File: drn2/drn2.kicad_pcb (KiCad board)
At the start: 2 copper layers, 123 x 89 mm, 60 parts, among them J1 Conn_01x03_Socket, J12 Conn_01x03_Socket, J13 Conn_01x03_Socket, J14GND1 Conn_01x03_Socket, J15VBECOUT1 Conn_01x03_Socket, J16 Conn_01x03_Socket, J2 Raspberry_Pi_2_3, J3 Conn_01x03_Socket, J3_F1_BEC_OUT1 Conn_01x02_Pin, J3_F2_BAT1 Conn_01x02_Pin, J4 Conn_01x03_Socket, J4_M0_MOT0 Conn_01x02_Pin, J4_M1_MOT1 Conn_01x02_Pin, J4_M2_MOT2 Conn_01x02_Pin, J4_M3_MOT3 Conn_01x02_Pin, J4_M4_BEC_IN1 Conn_01x02_Pin, J5 Conn_01x12_Socket, J6 Conn_01x08_Socket, J7 Conn_01x03_Socket, J8 Conn_01x03_Socket, U1 LSM9DS1, Y1 TestPoint

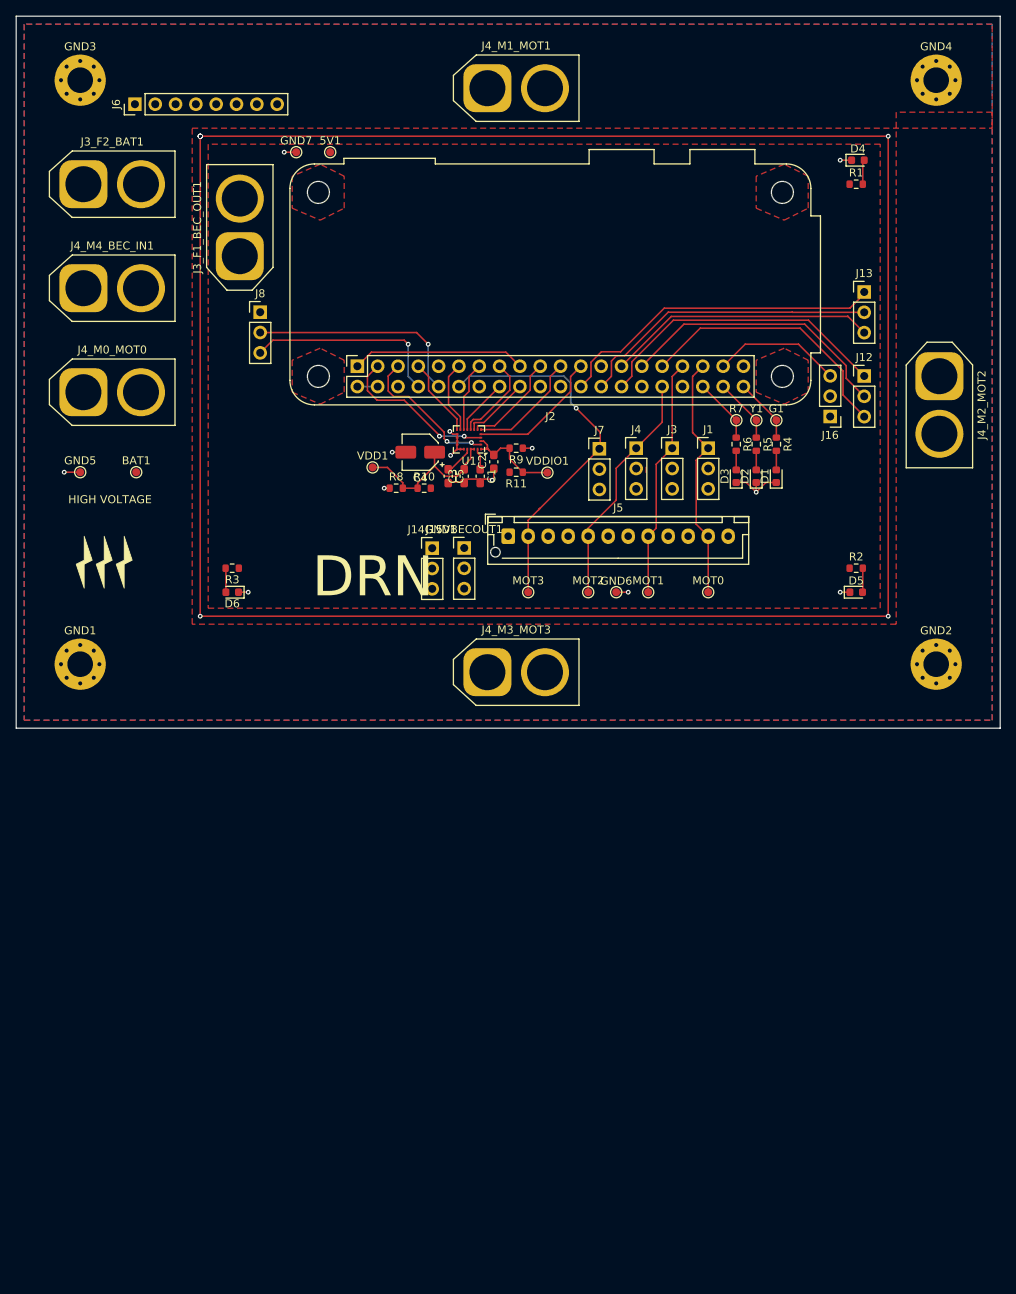
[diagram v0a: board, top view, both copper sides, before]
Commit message: feat: drn pcb v3 almost done
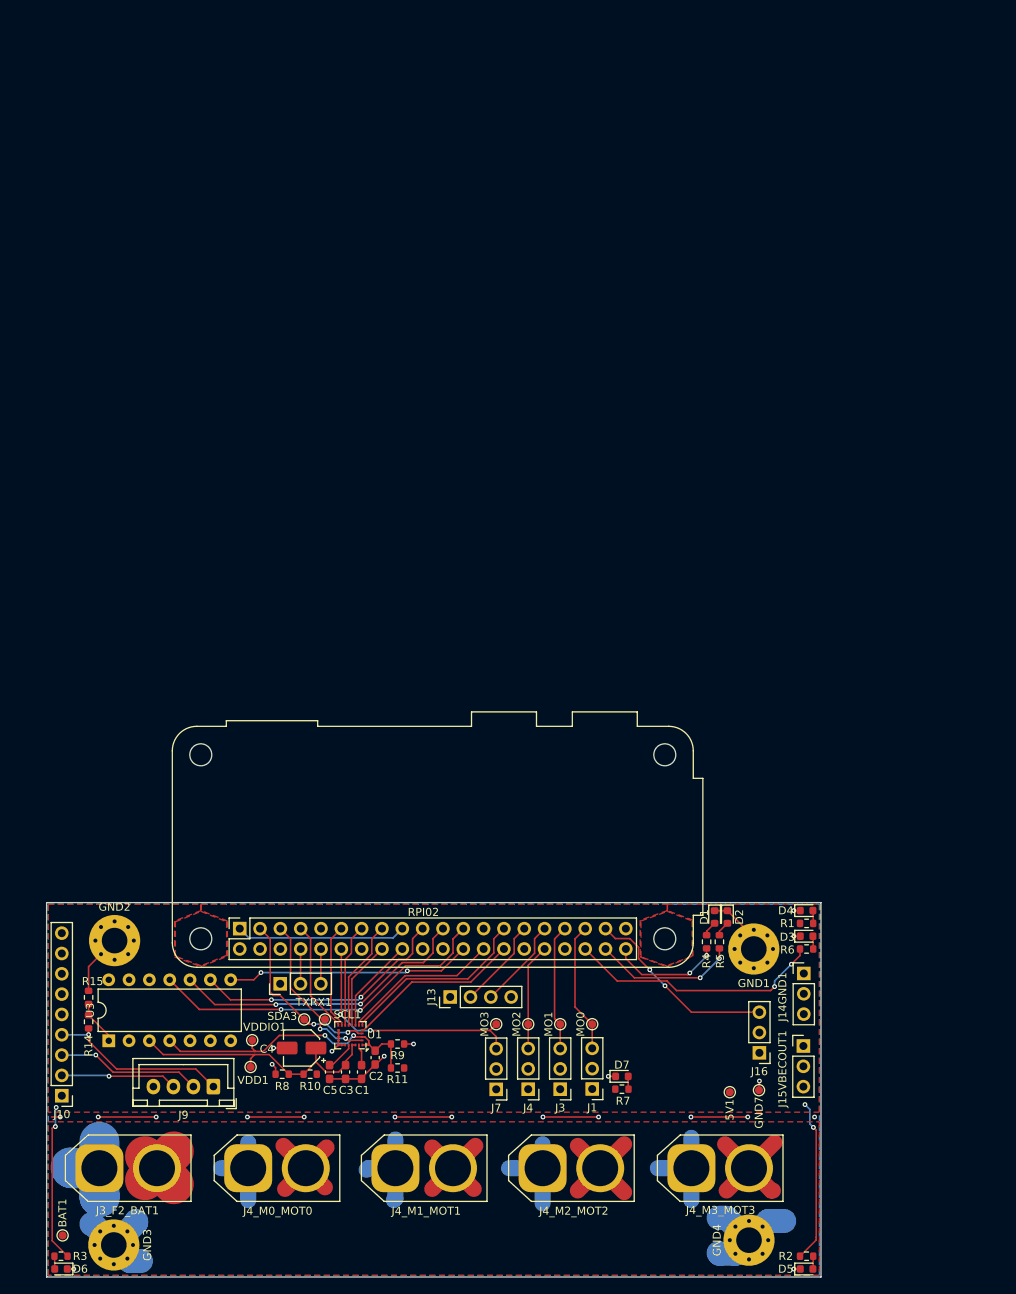
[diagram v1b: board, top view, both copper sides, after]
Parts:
- removed G1, GND5, GND6, MOT0, MOT1, MOT2, MOT3, Y1: TestPoint, TestPoint:TestPoint_Pad_D1.0mm
- removed J12, J8: Conn_01x03_Socket, Connector_PinHeader_2.54mm:PinHeader_1x03_P2.54mm_Vertical
- removed J2: Raspberry_Pi_2_3, Module:Raspberry_Pi_Zero_Socketed_THT_FaceDown_MountingHoles
- removed J3_F1_BEC_OUT1, J4_M4_BEC_IN1: Conn_01x02_Pin, Connector_AMASS:AMASS_XT60-F_1x02_P7.20mm_Vertical
- removed J5: Conn_01x12_Socket, Connector_JST:JST_XH_B12B-XH-AM_1x12_P2.50mm_Vertical
- removed J6: Conn_01x08_Socket, Connector_PinHeader_2.54mm:PinHeader_1x08_P2.54mm_Vertical
- added D7: LEDI, LED_SMD:LED_0603_1608Metric, F.Cu at (134.7, 158.5)
- added J10: Conn_01x09_Socket, Connector_PinHeader_2.54mm:PinHeader_1x09_P2.54mm_Vertical, F.Cu at (64.7, 160.9)
- added J9: Conn_01x04_Pin, Connector_JST:JST_XH_B4B-XH-A_1x04_P2.50mm_Vertical, F.Cu at (83.7, 159.8)
- added MO0: TestPoint, TestPoint:TestPoint_Pad_D1.0mm, F.Cu at (131.0, 152.0)
- added MO1: TestPoint, TestPoint:TestPoint_Pad_D1.0mm, F.Cu at (127.0, 152.0)
- added MO2: TestPoint, TestPoint:TestPoint_Pad_D1.0mm, F.Cu at (123.0, 152.0)
- added MO3: TestPoint, TestPoint:TestPoint_Pad_D1.0mm, F.Cu at (119.0, 152.0)
- added R14: 300K, Resistor_SMD:R_0603_1608Metric, F.Cu at (68.0, 151.7)
- added R15: 100k, Resistor_SMD:R_0603_1608Metric, F.Cu at (68.0, 148.7)
- added RPI02: Raspberry_Pi_2_3, Module:Raspberry_Pi_Zero_Socketed_THT_FaceDown_MountingHoles, F.Cu at (86.9, 140.1)
- added SCL1: TestPoint, TestPoint:TestPoint_Pad_D1.0mm, F.Cu at (97.6, 151.4)
- added SDA3: TestPoint, TestPoint:TestPoint_Pad_D1.0mm, F.Cu at (95.0, 151.4)
- added TXRX1: Conn_01x03_Socket, Connector_PinHeader_2.54mm:PinHeader_1x03_P2.54mm_Vertical, F.Cu at (92.0, 146.9)
- added U3: MCP3004, Package_DIP:DIP-14_W7.62mm, F.Cu at (70.6, 154.1)
- J13: value Conn_01x03_Socket -> Conn_01x04_Socket; footprint Connector_PinHeader_2.54mm:PinHeader_1x03_P2.54mm_Vertical -> Connector_PinHeader_2.54mm:PinHeader_1x04_P2.54mm_Vertical
- R7: value TestPoint -> 130; footprint TestPoint:TestPoint_Pad_D1.0mm -> Resistor_SMD:R_0603_1608Metric
- moved GND4 146.9 mm to (150.6, 179.0)
- moved GND3 145.7 mm to (71.2, 179.6)
- moved J4_M1_MOT1 135.5 mm to (106.4, 170.0)
- moved GND7 130.7 mm to (151.8, 160.2)
- moved 5V1 127.7 mm to (148.2, 160.5)
- moved J3_F2_BAT1 123.0 mm to (69.4, 170.0)
- moved J4_M2_MOT2 110.7 mm to (124.8, 170.0), turned to 0 degrees
- moved GND2 108.4 mm to (71.3, 141.6)
- moved J13 102.2 mm to (113.2, 148.6), turned to 90 degrees
- moved J4_M0_MOT0 99.2 mm to (88.0, 170.0)
- moved BAT1 95.8 mm to (64.8, 178.4)
- moved D4 94.0 mm to (157.8, 137.8)
- moved R1 92.6 mm to (157.8, 139.4)
- moved GND1 91.4 mm to (151.2, 142.6)
- moved R3 88.6 mm to (64.6, 181.0)
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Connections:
- J1 pad 1: Net-(J1-Pin_1) -> GND
- J1 pad 3: GND -> Net-(J1-Pin_3)
- J13 pad 1: Net-(J13-Pin_1) -> GND
- J3 pad 1: Net-(J2-PWM1/GPIO13) -> GND
- J3 pad 3: GND -> Net-(J3-Pin_3)
- J4 pad 1: Net-(J2-PWM0/GPIO12) -> GND
- J4 pad 3: GND -> Net-(J4-Pin_3)
- J7 pad 1: Net-(J2-GPIO18/PWM0) -> GND
- J7 pad 3: GND -> Net-(J7-Pin_3)
- R6 pad 1: Net-(J2-GPIO16) -> Net-(RPI02-GPIO16)
- R7 pad 1: Net-(J2-GPIO16) -> /5V
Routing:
- net GND: track 31.7 -> 303.7 mm, vias 22 -> 23
- net /11.1: track 0.00 -> 144.2 mm
- net Net-(J2-GPIO18/PWM0): track 46.2 -> 0.00 mm, vias 1 -> 0
- net Net-(RPI02-SCLK0/GPIO11): track 0.00 -> 43.6 mm, vias 0 -> 2
- net Net-(J13-Pin_1): track 41.3 -> 0.00 mm
- net Net-(RPI02-MISO0/GPIO9): track 0.00 -> 37.9 mm, vias 0 -> 2
- net /5V: track 3.17 -> 40.9 mm, vias 0 -> 4
- net Net-(J12-Pin_1): track 37.7 -> 0.00 mm
- net Net-(J12-Pin_2): track 34.6 -> 0.00 mm
- net Net-(J12-Pin_3): track 33.6 -> 0.00 mm
- net Net-(RPI02-MOSI0/GPIO10): track 0.00 -> 32.3 mm, vias 0 -> 2
- net Net-(RPI02-GPIO16): track 0.00 -> 32.1 mm, vias 0 -> 2
- net Net-(J7-Pin_3): track 0.00 -> 31.5 mm, vias 0 -> 2
- net Net-(RPI02-~{CE0}/GPIO8): track 0.00 -> 30.7 mm, vias 0 -> 2
- net Net-(J1-Pin_1): track 30.6 -> 0.00 mm
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- added copper zone on In1.Cu, net /11.1
- added copper zone on In1.Cu, net /5V
- added copper zone on In2.Cu, net GND
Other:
- board size 123 x 89 mm -> 96.8 x 46.8 mm
- copper layers 2 -> 4
- board text removed: "DRN"
- board text removed: "HIGH VOLTAGE"
